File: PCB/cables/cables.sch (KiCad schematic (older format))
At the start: 26 parts

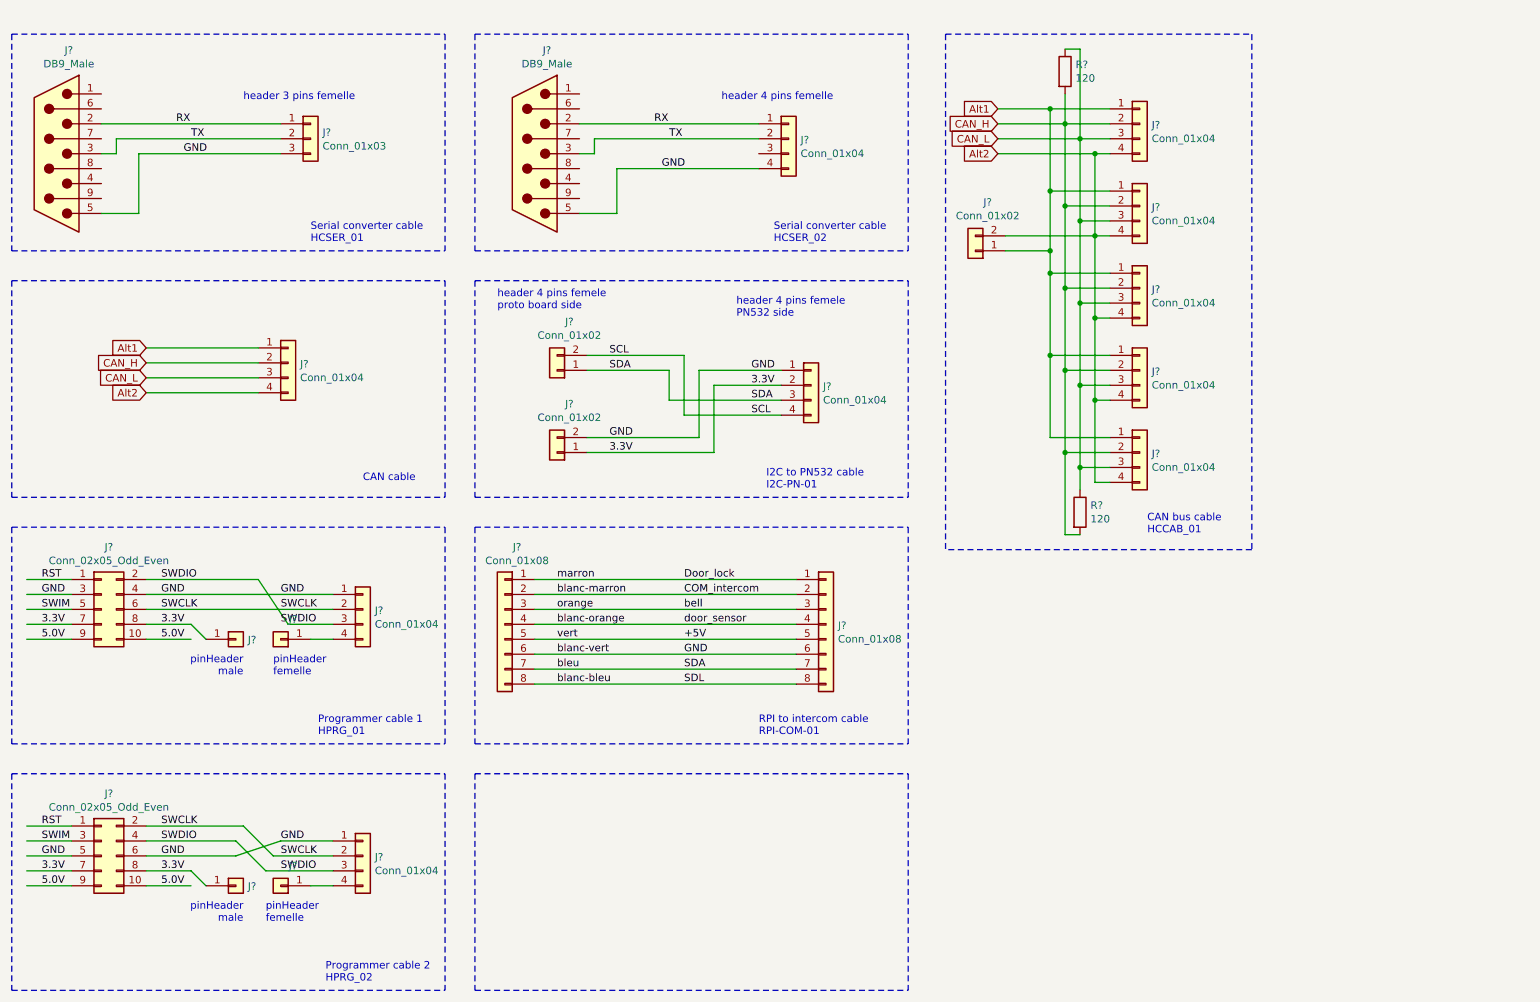
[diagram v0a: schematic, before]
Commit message: update PCB
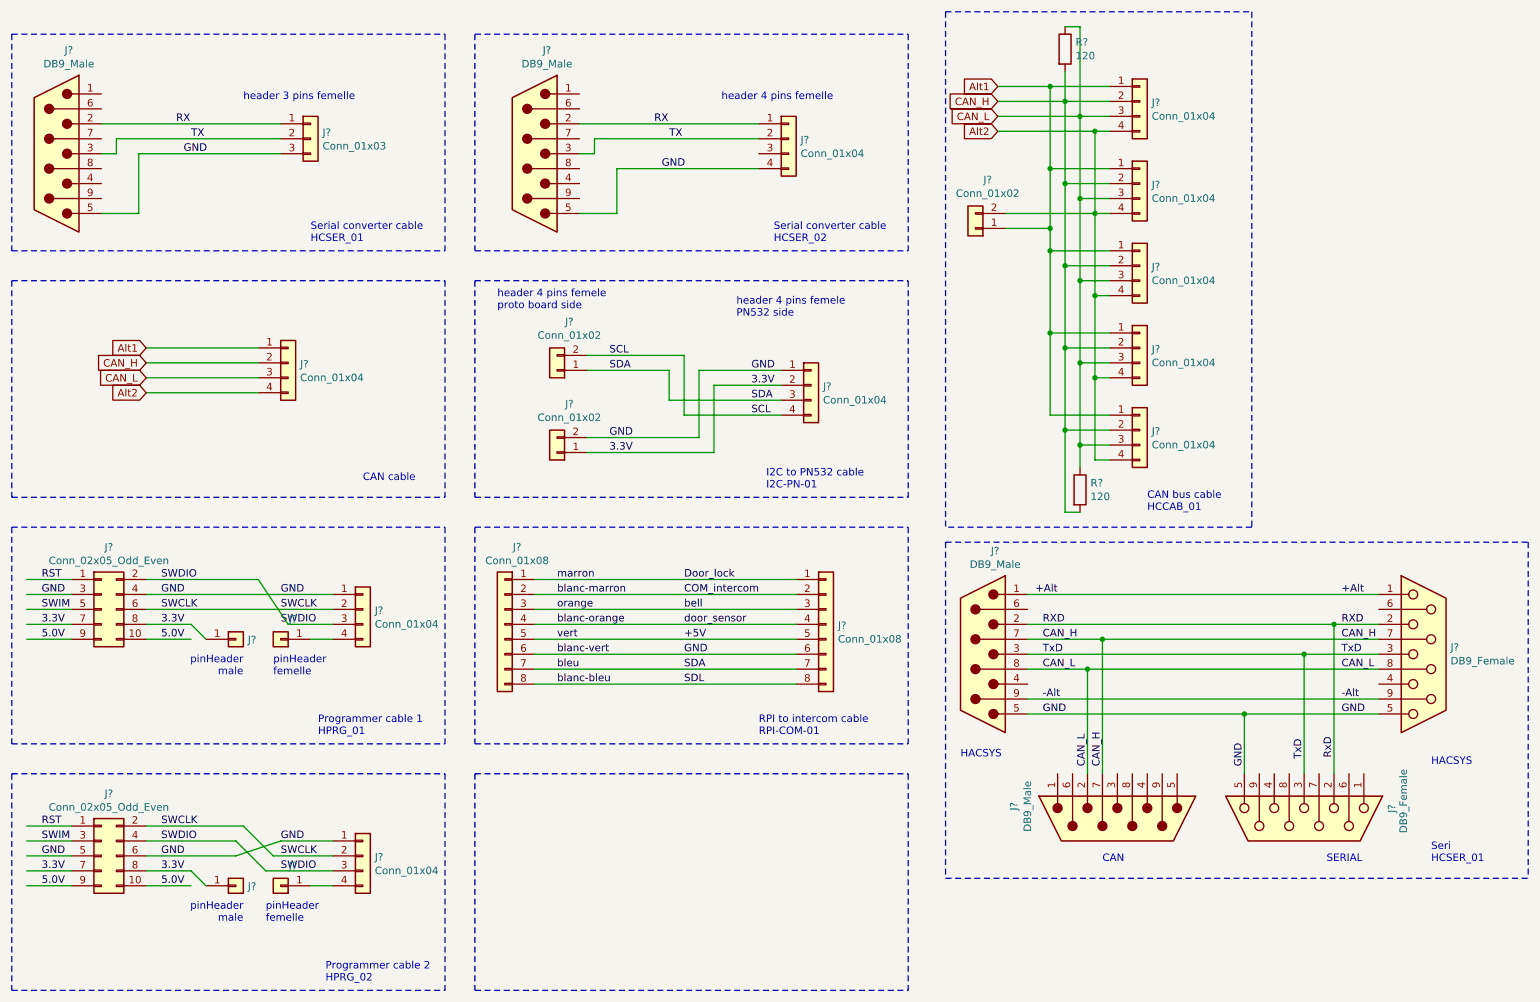
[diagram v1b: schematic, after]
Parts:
- added J? (x2): DB9_Male, symbol Connector:DB9_Male
- added J? (x2): DB9_Female, symbol Connector:DB9_Female
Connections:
- net labels added: +Alt, -Alt, RXD, RxD, TxD
- wire segments 119 -> 136
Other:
- note added: "CAN"
- note added: "HACSYS"
- note added: "SERIAL"
- note added: "Seri\nHCSER_01"
- moved on the sheet: J?, R?
